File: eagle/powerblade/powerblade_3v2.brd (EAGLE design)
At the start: 25.4 x 25.4 mm, 79 parts, among them J1 JTAG_14PIN_IDC-ND, J2 AC_INF41, J4 TC2030-JLINK-NL, Q1 NTS4173, Q4 2SK1829, U1 TPS62122, U2 MCP6V3, U3 MSP430FR5738, U4 NRF51822QF, U6 MAX9910, U7 OPA2369, X1 16MHz, X3 32.768kHz, Y1 UREACH_XTEND

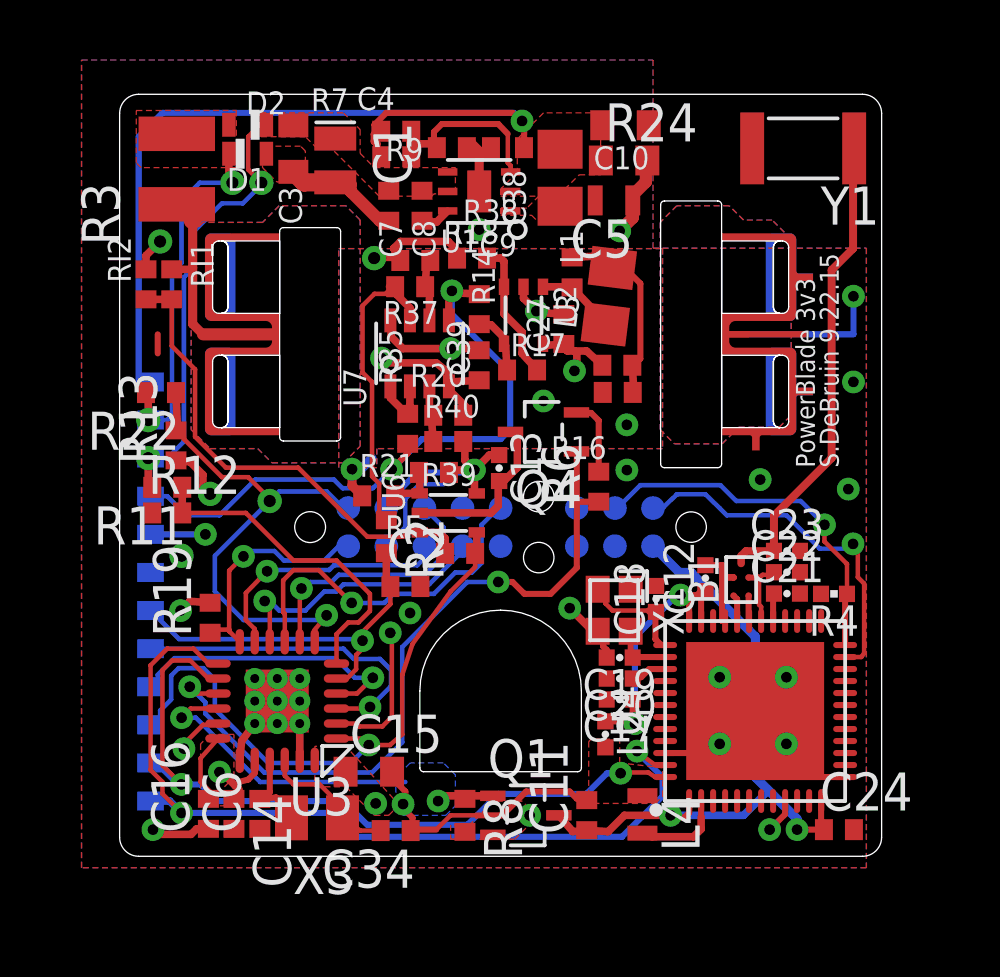
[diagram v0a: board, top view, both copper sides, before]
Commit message: updated board? I hope i dont get conflicts
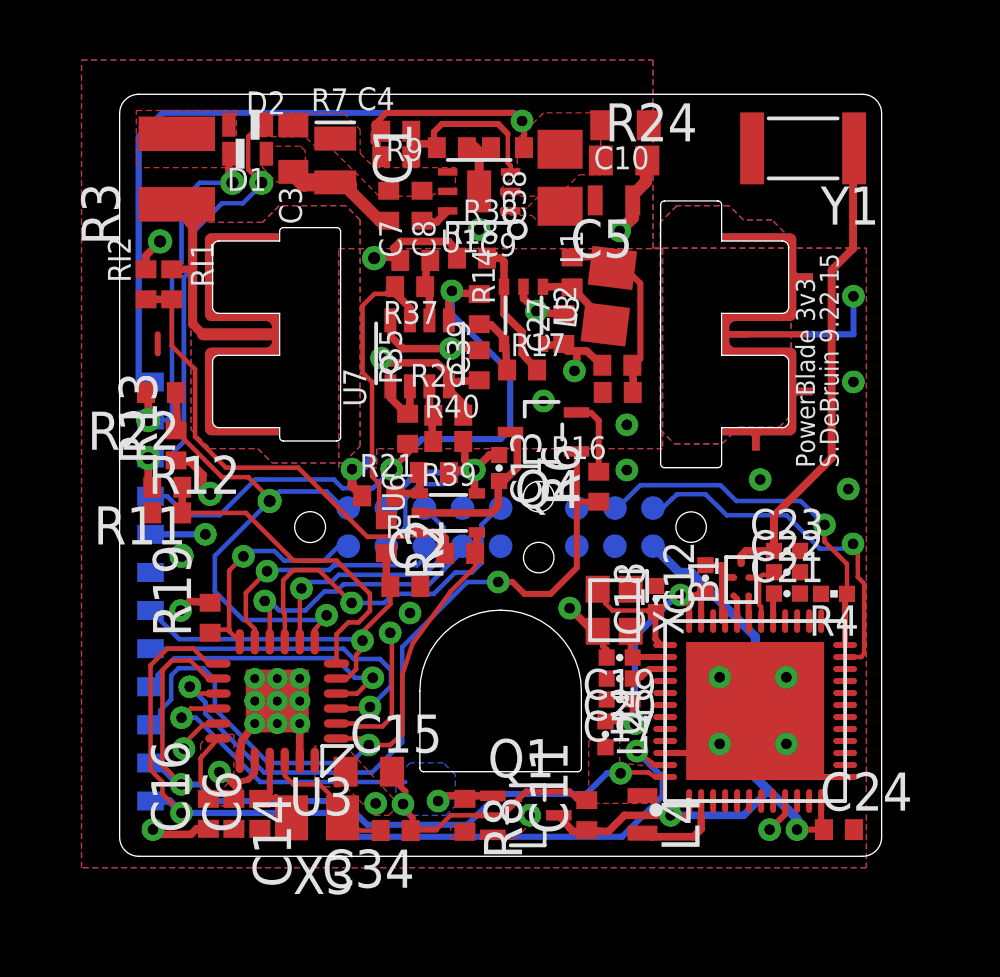
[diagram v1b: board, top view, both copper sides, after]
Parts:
- J2: value AC_INF41 -> AC_INF45; device powerfilm:AC3_F41 -> powerfilm:AC3_F45
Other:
- outline, holes or cut-outs redrawn
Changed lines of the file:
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@@
 <attribute name="DIGIKEY" value="490-4025-1-ND" x="4.727575" y="-16.002" size="1.778" layer="27" rot="R270" display="off"/>
 </element>
-<element name="J2" library="powerfilm" package="AC3_F41" value="AC_INF41" x="0" y="0">
+<element name="J2" library="powerfilm" package="AC3_F45" value="AC_INF45" x="0" y="0">
 <attribute name="DIGIKEY" value="ED1649-ND" x="0" y="0" size="1.778" layer="27" display="off"/>
 <attribute name="DIGIKEY_2" value="ED1649-ND" x="0" y="0" size="1.778" layer="27" display="off"/>
